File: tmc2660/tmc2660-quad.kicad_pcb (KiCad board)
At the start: 4 copper layers, 125 x 40 mm, 81 parts, among them J1 Power, J100 0R, J2 DataIn, J200 0R, J300 0R, J400 0R, M0 Mount, M1 Mount, M100 Mount, M101 Mount, M200 Mount, M201 Mount, M300 Mount, M301 Mount, M400 Mount, M401 Mount, P100 Motor, P200 Motor, P300 Motor, P400 Motor, U100 TMC2660, U200 TMC2660, U300 TMC2660, U400 TMC2660

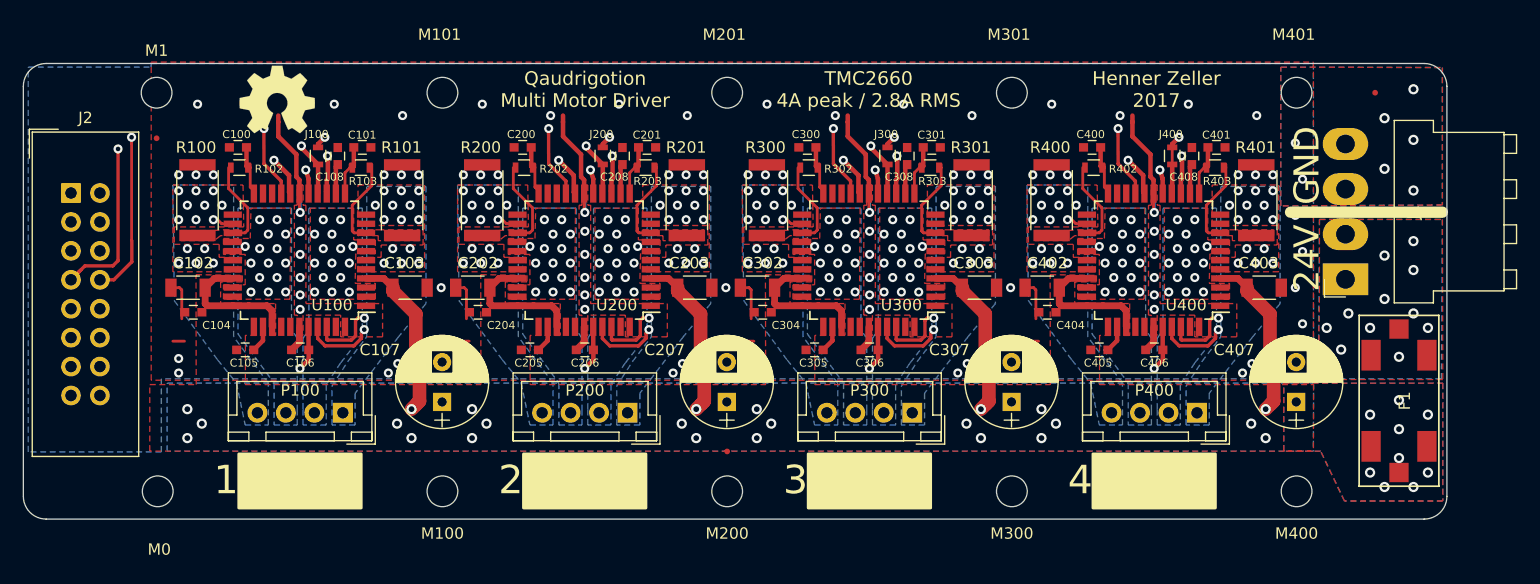
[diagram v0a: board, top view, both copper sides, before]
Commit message: Merge new template + baseline.
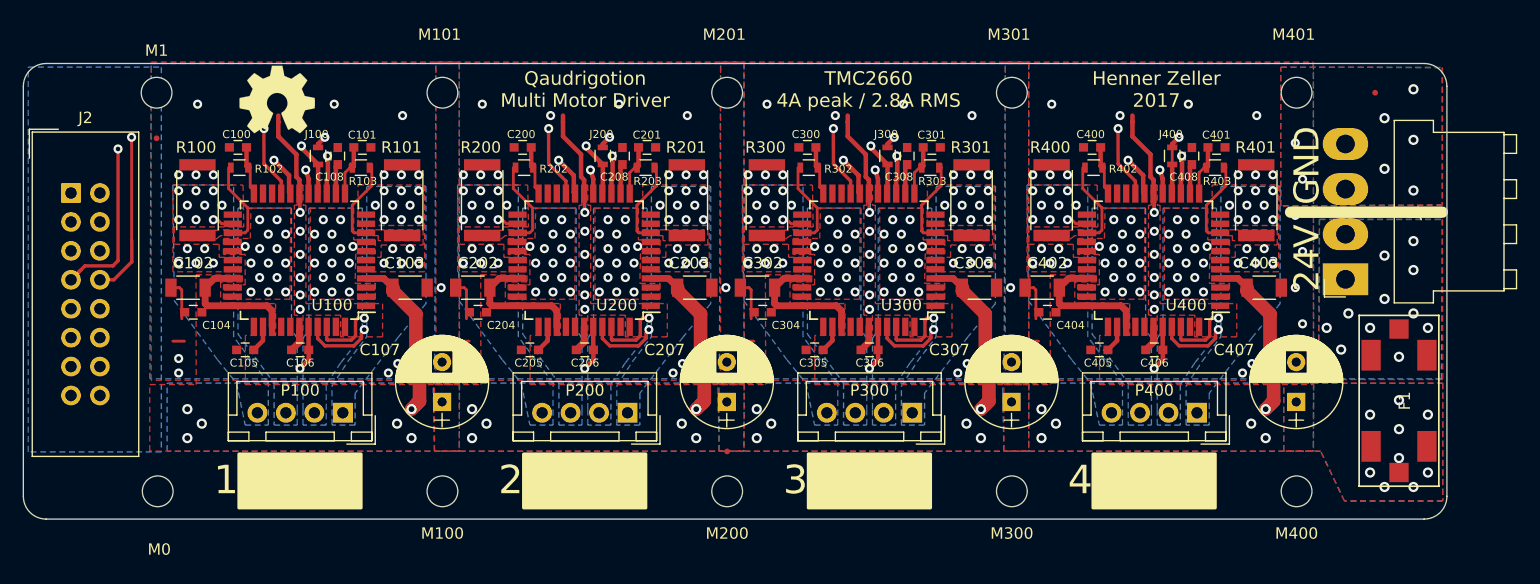
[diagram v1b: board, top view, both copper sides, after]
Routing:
- net DIR4: track 110.4 -> 111.0 mm
